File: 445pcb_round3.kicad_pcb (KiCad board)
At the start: 2 copper layers, 83.5 x 51 mm, 45 parts, among them J1 LED, J10 AVR-ISP-6, J11 SG1, J13 LED, J19 Conn_01x04_Pin, J2 LED, J3 LED, J4 SG3, J5 SG4, J6 SG5, J7 SG6, J8 SG1, J9 SG2, SW1 SW_SPST, U1 ICM-20948, U3 ATmega328P-A, U6 LM358DT, U7 LM358DT

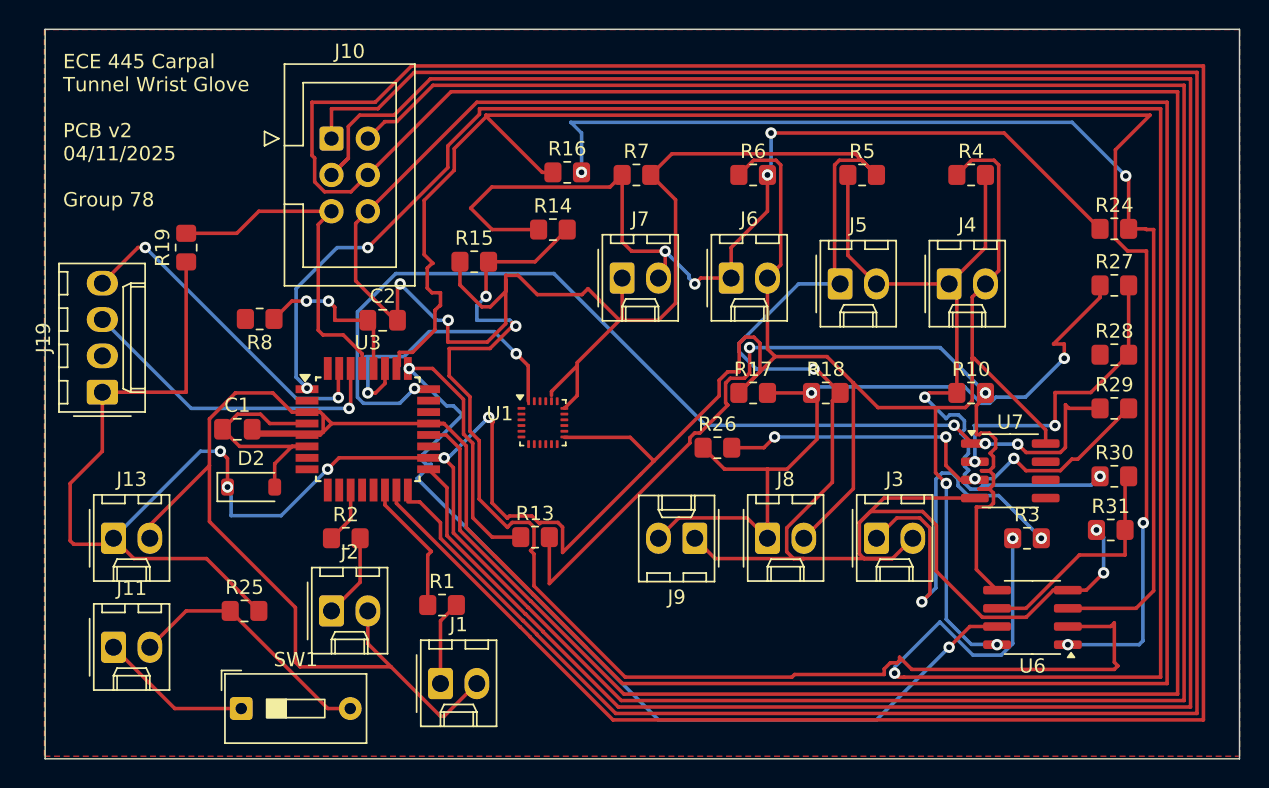
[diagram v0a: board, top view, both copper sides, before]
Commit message: Add files via upload
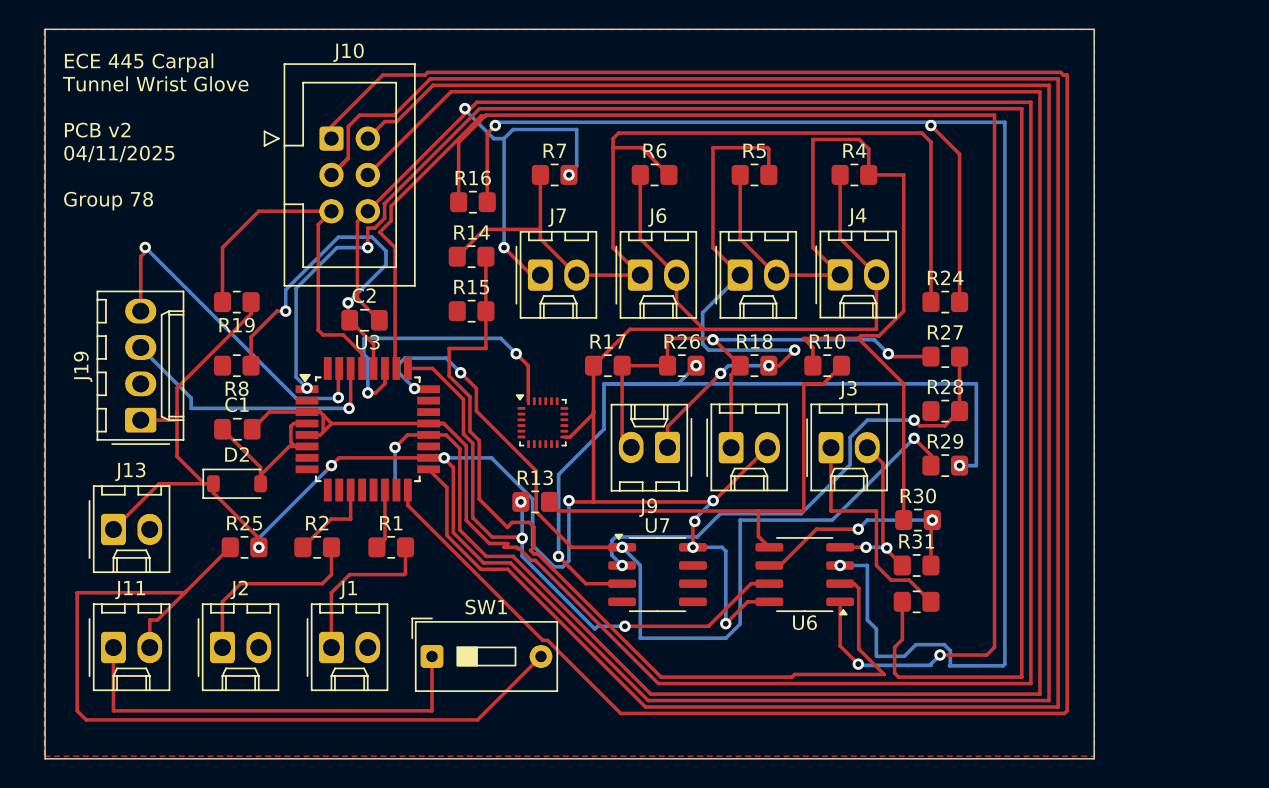
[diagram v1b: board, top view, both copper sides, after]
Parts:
- moved U7 25.7 mm to (119.3, 71.1)
- moved U6 16.2 mm to (129.6, 71.1)
- moved R30 14.1 mm to (137.5, 67.3)
- moved SW1 13.8 mm to (103.5, 76.8)
- moved R31 13.8 mm to (137.4, 70.5)
- moved R24 12.9 mm to (139.4, 52.1)
- moved R27 12.8 mm to (139.4, 55.9)
- moved R29 12.5 mm to (139.4, 63.5)
- moved R28 12.5 mm to (139.4, 59.7)
- moved R17 10.3 mm to (115.8, 56.5)
- moved R10 10.2 mm to (131.2, 56.5)
- moved R3 8.90 mm to (137.4, 73.0)
- moved R4 8.16 mm to (133.1, 43.2)
- moved J2 8.04 mm to (88.9, 76.2)
- moved J1 8.03 mm to (96.5, 76.2)
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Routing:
- net MOSI: track 347.2 -> 150.8 mm, vias 0 -> 1
- net GND: track 434.7 -> 246.0 mm, vias 5 -> 9
- net +5V: track 384.5 -> 300.1 mm, vias 7 -> 8
- net Net-(J11-Pin_2): track 17.9 -> 60.0 mm
- net Vdiff1: track 79.1 -> 42.0 mm, vias 2 -> 3
- net Net-(U3-PD3): track 151.1 -> 118.6 mm, vias 4 -> 2
- net Net-(U6-IN2+): track 64.5 -> 33.0 mm, vias 2 -> 0
- net Net-(U6-IN1+): track 81.5 -> 111.6 mm, vias 2 -> 3
- net Net-(U6-IN1-): track 91.4 -> 63.7 mm, vias 2 -> 0
- net Net-(U7-IN1+): track 33.2 -> 58.5 mm, vias 4 -> 3
- net Net-(J11-Pin_1): track 10.7 -> 30.5 mm
- net MISO: track 170.4 -> 151.6 mm
- net SCK: track 171.8 -> 153.3 mm
- net V+: track 56.4 -> 38.7 mm
- net IMU_OUT: track 11.6 -> 25.6 mm
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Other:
- board size 83.5 x 51 mm -> 73.3 x 51 mm
